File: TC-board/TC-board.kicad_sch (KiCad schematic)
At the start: 6 parts, among them J1 DB15_Female, J3 PCIE-LP-01-01-F-DV-A-TR

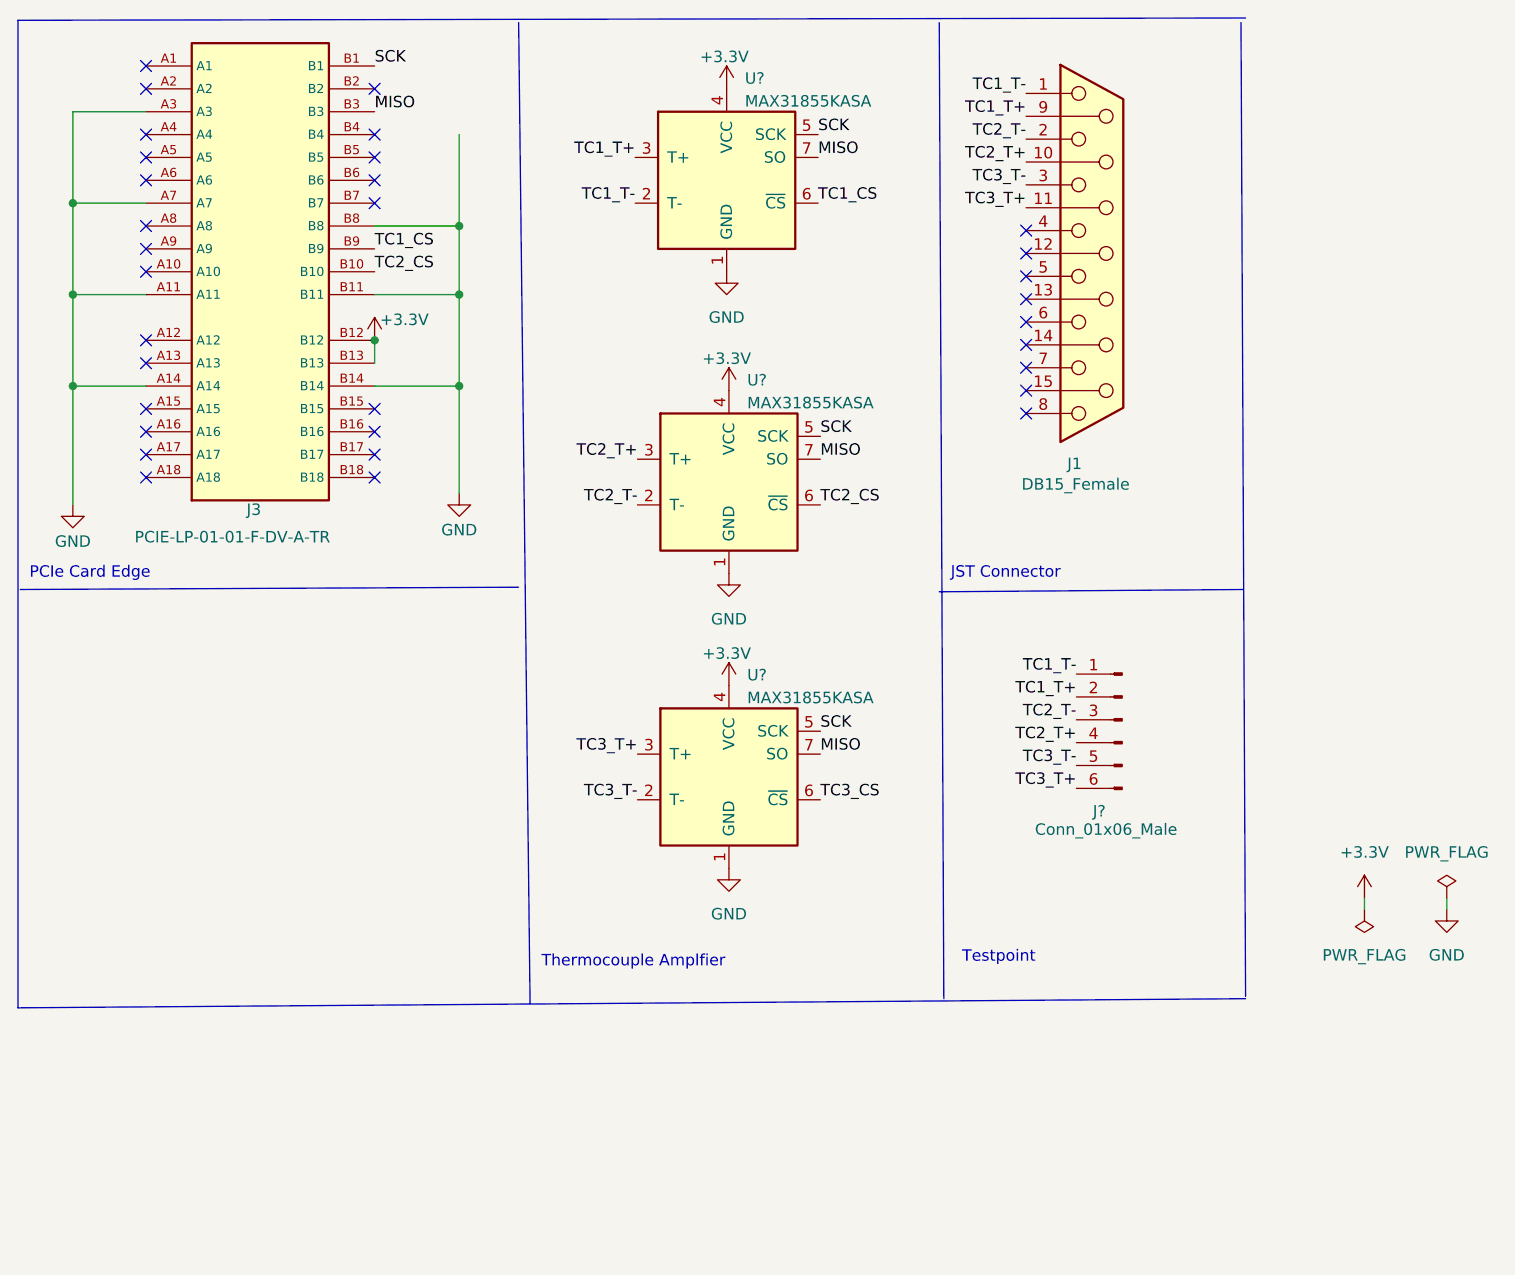
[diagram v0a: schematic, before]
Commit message: Updated schematics of TC,PT
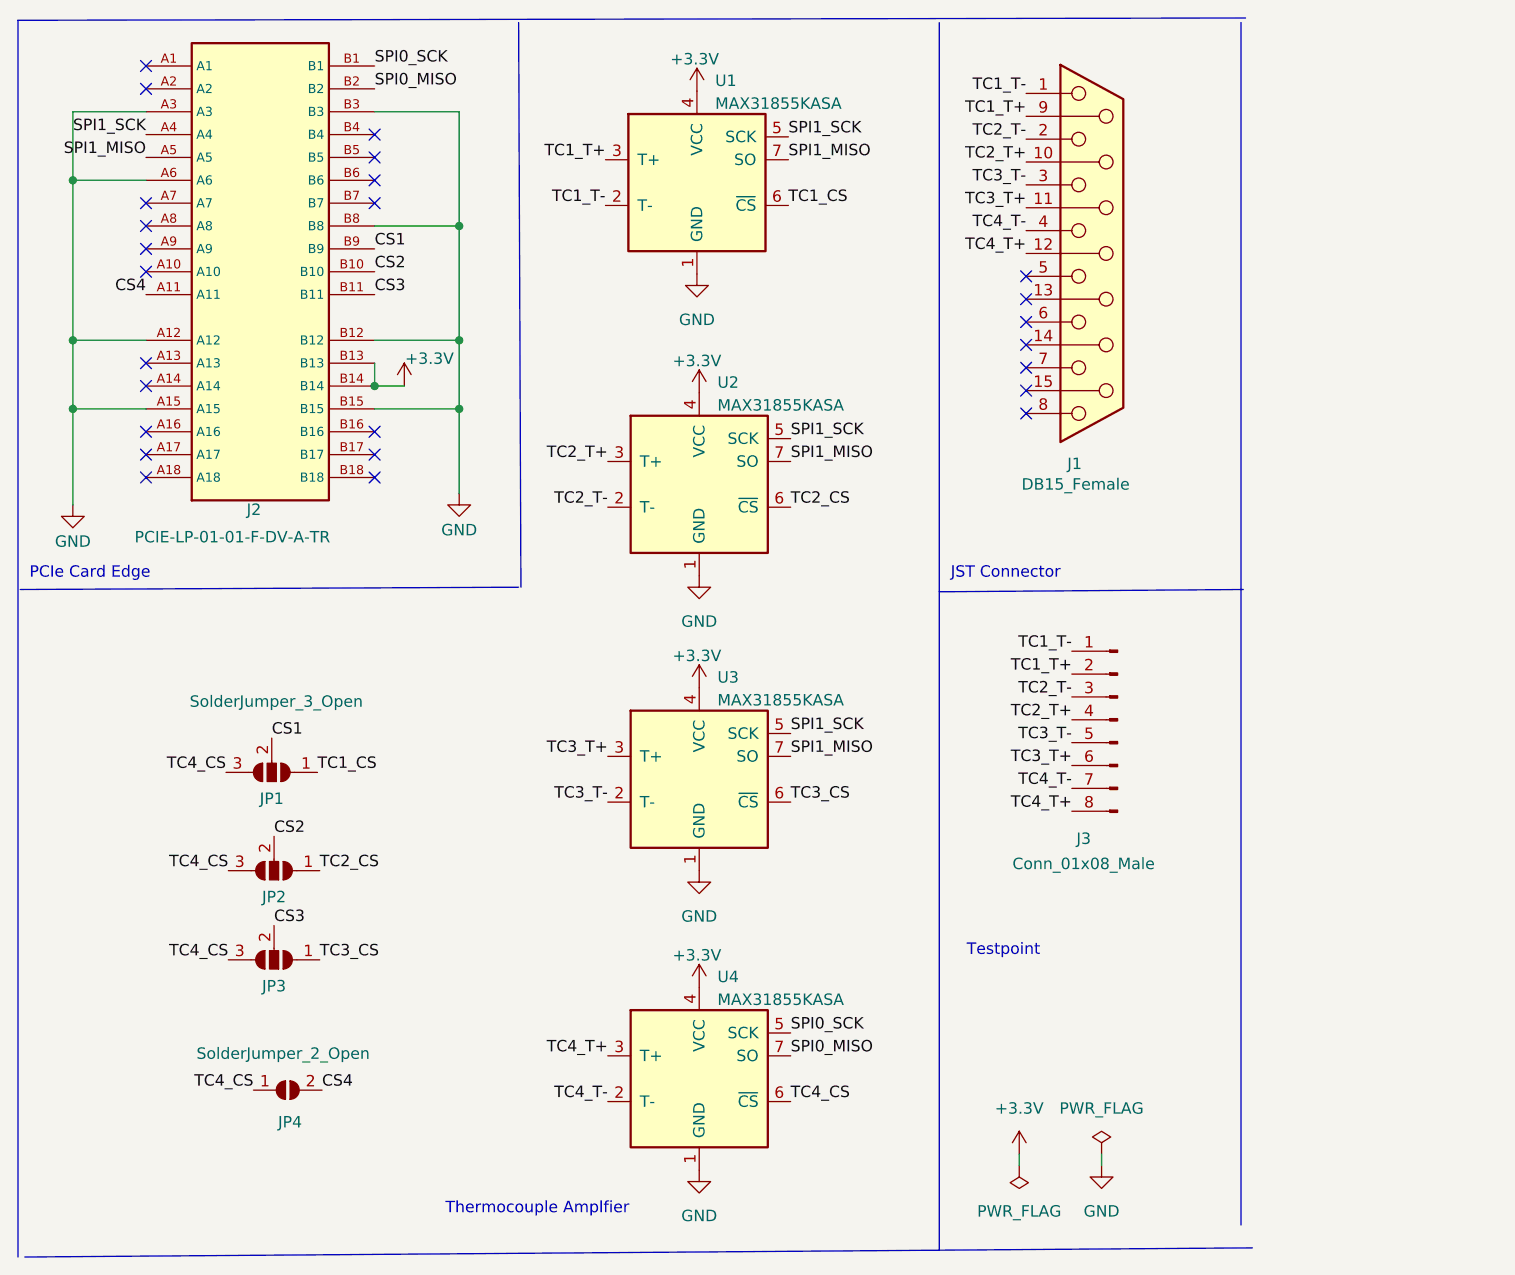
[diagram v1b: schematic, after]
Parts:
- removed J?: Conn_01x06_Male, symbol Connector:Conn_01x06_Male
- added J3: Conn_01x08_Male, Connector_PinHeader_2.54mm:PinHeader_1x08_P2.54mm_Vertical, symbol Connector:Conn_01x08_Male
- added JP1, JP2, JP3: SolderJumper_3_Open, Jumper:SolderJumper-3_P2.0mm_Open_TrianglePad1.0x1.5mm, symbol Jumper:SolderJumper_3_Open
- added JP4: SolderJumper_2_Open, Jumper:SolderJumper-2_P1.3mm_Open_TrianglePad1.0x1.5mm, symbol Jumper:SolderJumper_2_Open
- added U4: MAX31855KASA, MAX31855_Breakout:MAX31855_Breakout, symbol Sensor_Temperature:MAX31855KASA
- U1, U2, U3: renamed from U?; footprint Package_SO:SOIC-8_3.9x4.9mm_P1.27mm -> MAX31855_Breakout:MAX31855_Breakout
- renumbered J3 to J2
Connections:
- net +3.3V: now also J2.B14, U4.4 (VCC); no longer J2.B12
- net GND: now also J2.A12, J2.A15, J2.A6, J2.B12, J2.B15, J2.B3, U4.1 (GND); no longer J2.A11, J2.A14, J2.A7, J2.B11, J2.B14
- net TC1_CS: now also JP1.1 (A); no longer J2.B9
- net TC1_T+: now also J3.2 (Pin_2)
- net TC1_T-: now also J3.1 (Pin_1)
- net TC2_CS: now also JP2.1 (A); no longer J2.B10
- net TC2_T+: now also J3.4 (Pin_4)
- net TC2_T-: now also J3.3 (Pin_3)
- net TC3_CS: now also JP3.1 (A)
- net TC3_T+: now also J3.6 (Pin_6)
- net TC3_T-: now also J3.5 (Pin_5)
- net SPI1_SCK: now reaches J2.A4
- net SPI1_SCK: now also U1.5 (SCK), U2.5 (SCK), U3.5 (SCK)
- net SPI1_MISO: now reaches J2.A5
- net SPI1_MISO: now also U1.7 (SO), U2.7 (SO), U3.7 (SO)
- net SPI0_MISO: now reaches J2.B2
- net SPI0_MISO: now also U4.7 (SO)
- net TC4_T+: now reaches J1.12 (P12)
- net TC4_T+: now also J3.8 (Pin_8), U4.3 (T+)
- net TC4_T-: now reaches J1.4
- net TC4_T-: now also J3.7 (Pin_7), U4.2 (T-)
- removed net MISO: J2.B3, U1.7 (SO), U2.7 (SO), U3.7 (SO)
- removed net SCK: J2.B1, U1.5 (SCK), U2.5 (SCK), U3.5 (SCK)
- new net CS1: J2.B9, JP1.2 (C)
- new net CS2: J2.B10, JP2.2 (C)
- new net CS3: J2.B11, JP3.2 (C)
- new net CS4: J2.A11, JP4.2 (B)
- new net SPI0_SCK: J2.B1, U4.5 (SCK)
- new net TC4_CS: JP1.3 (B), JP2.3 (B), JP3.3 (B), JP4.1 (A), U4.6 (~{CS})
- no-connect marks 32 -> 25
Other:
- moved on the sheet: U1, U2, U3
